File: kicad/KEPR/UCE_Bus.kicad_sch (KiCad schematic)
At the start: 1 part, among them J11 10141995-005RLF

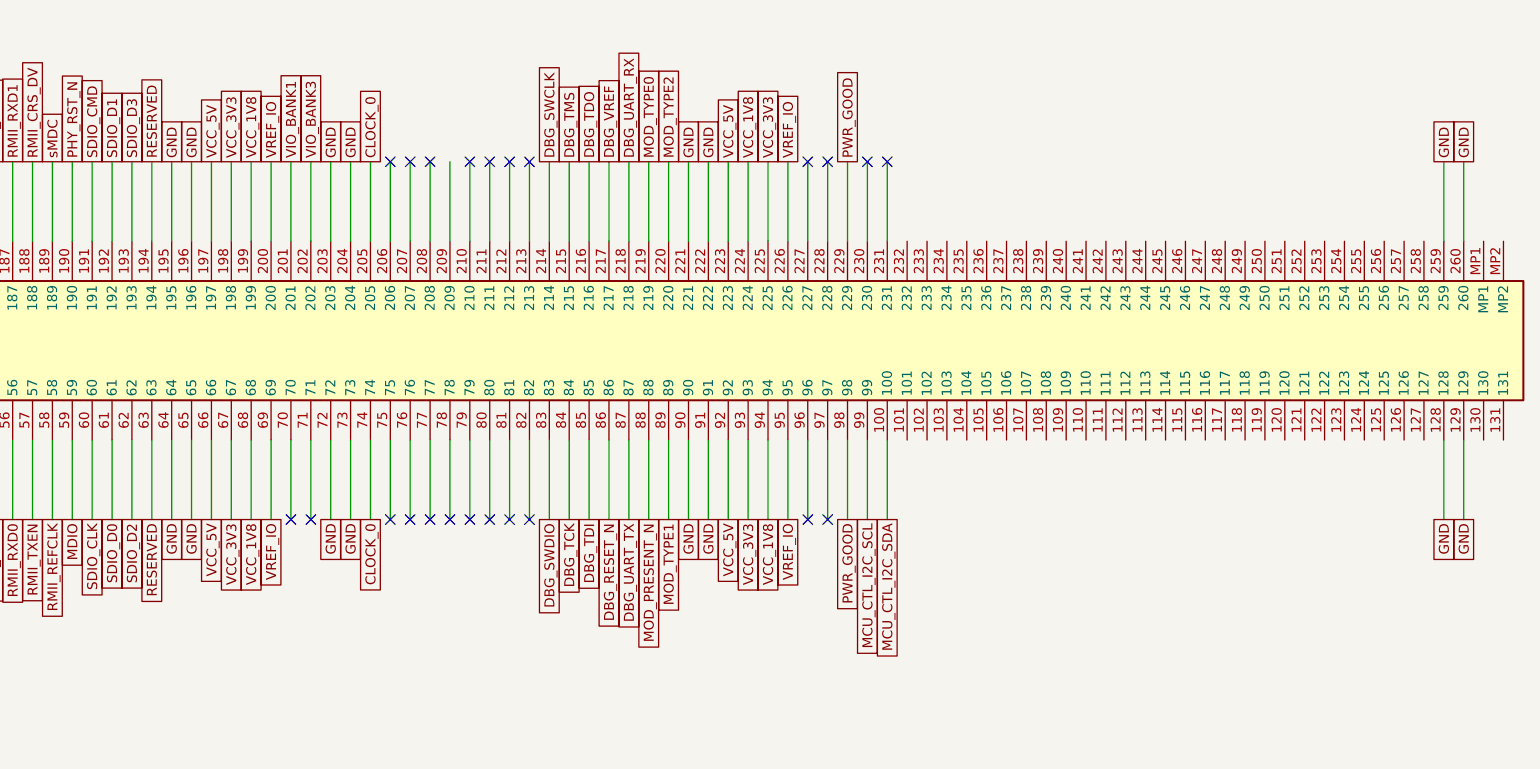
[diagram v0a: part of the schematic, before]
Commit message: mais ajustes de trilha.
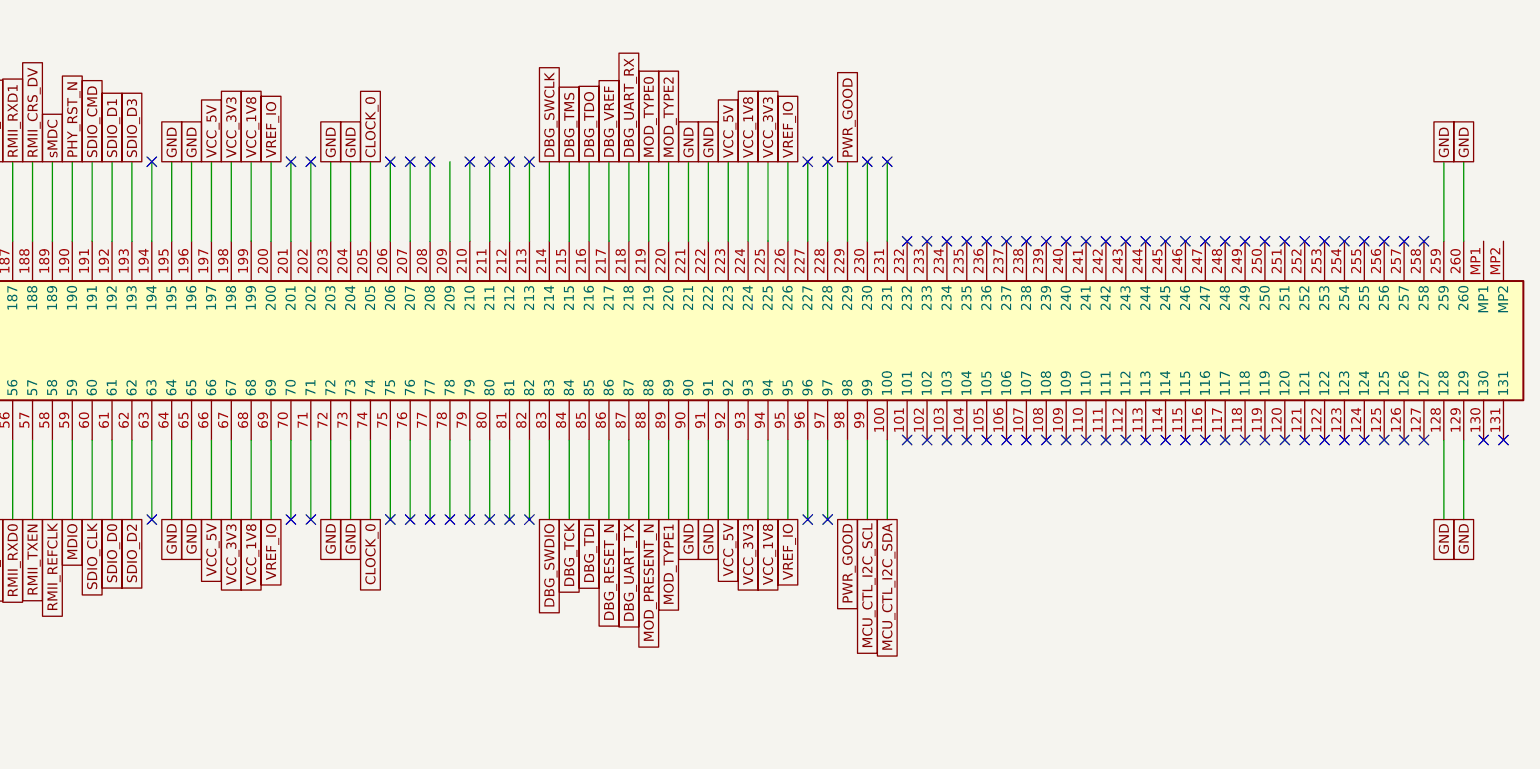
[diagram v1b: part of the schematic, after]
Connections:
- net RESERVED: no longer names the net of J11.194
- net RESERVED: no longer J11.63
- net VIO_BANK1: no longer names the net of J11.201
- net VIO_BANK3: no longer names the net of J11.202
- no-connect marks 27 -> 87
